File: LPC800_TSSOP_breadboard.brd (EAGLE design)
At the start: 30.5 x 17.8 mm, 16 parts, among them Q1 12MHz

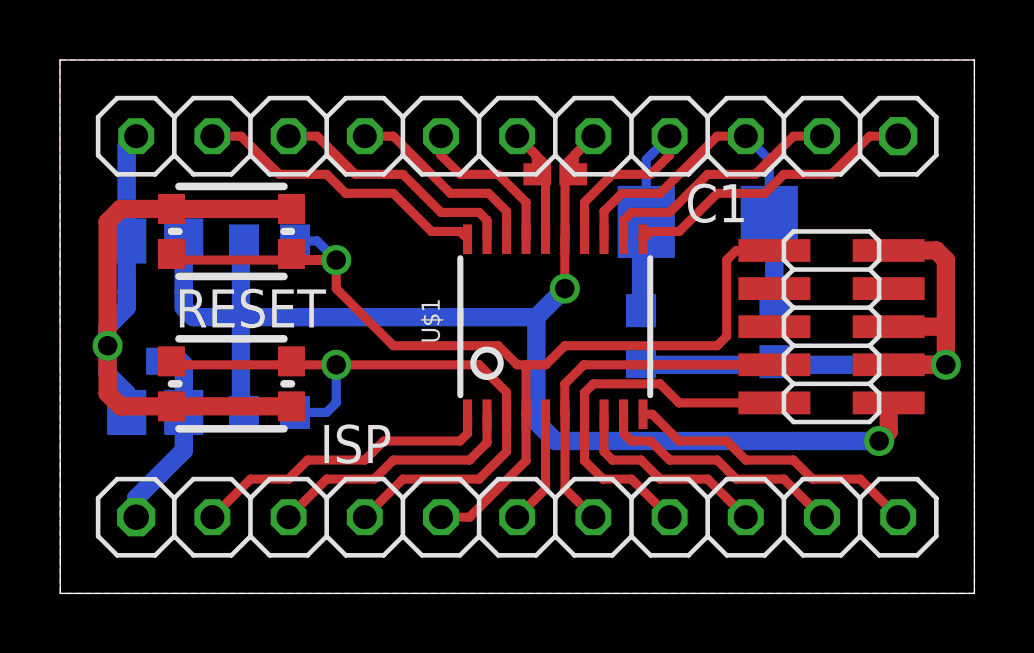
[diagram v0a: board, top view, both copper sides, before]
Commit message: * small updates
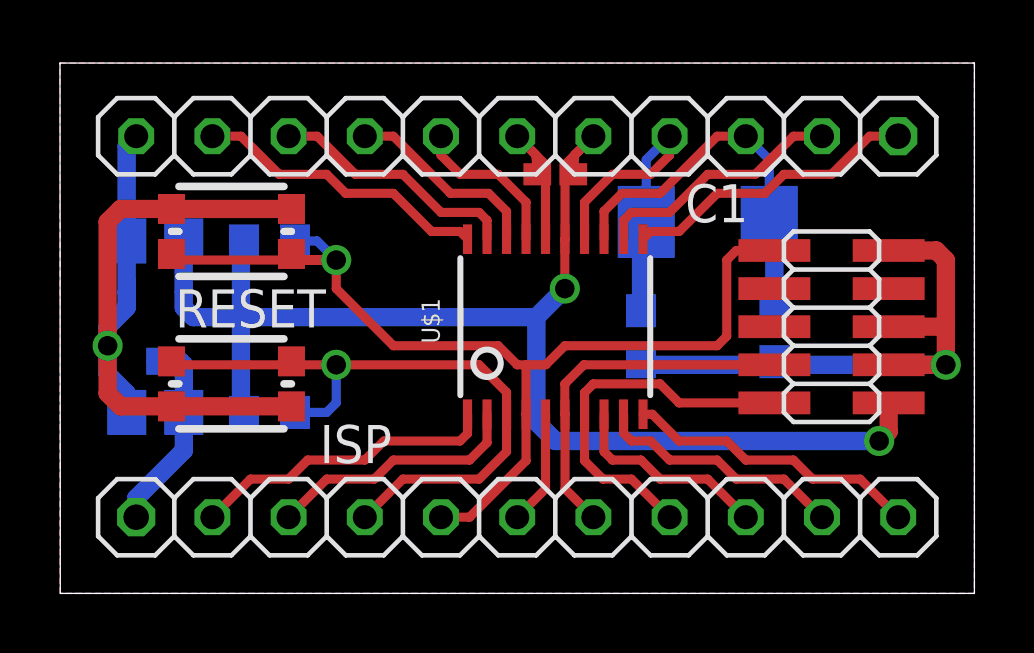
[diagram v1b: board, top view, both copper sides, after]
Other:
- board size 30.5 x 17.8 mm -> 30.5 x 17.7 mm
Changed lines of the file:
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@@
 <board>
 <plain>
-<wire x1="30.48" y1="0" x2="30.48" y2="17.78" width="0" layer="20"/>
-<wire x1="30.48" y1="17.78" x2="0" y2="17.78" width="0" layer="20"/>
-<wire x1="0" y1="17.78" x2="0.01" y2="0" width="0" layer="20"/>
+<wire x1="30.48" y1="0" x2="30.48" y2="17.6784" width="0" layer="20"/>
+<wire x1="30.48" y1="17.6784" x2="0" y2="17.6784" width="0" layer="20"/>
+<wire x1="0" y1="17.6784" x2="0.01" y2="0" width="0" layer="20"/>
 <wire x1="0.01" y1="0" x2="30.48" y2="0" width="0" layer="20"/>
 <wire x1="0" y1="0" x2="0" y2="17.6784" width="0.254" layer="102"/>
@@
 <wire x1="15.86" y1="14.62" x2="15.24" y2="15.24" width="0.3048" layer="1"/>
 <polygon width="0.254" layer="1">
-<vertex x="0" y="17.78"/>
-<vertex x="30.48" y="17.78"/>
+<vertex x="0" y="17.6784"/>
+<vertex x="30.48" y="17.6784"/>
 <vertex x="30.48" y="0"/>
 <vertex x="0" y="0"/>
 </polygon>
 <polygon width="0.254" layer="16">
-<vertex x="0" y="17.78"/>
-<vertex x="30.48" y="17.78"/>
+<vertex x="0" y="17.6784"/>
+<vertex x="30.48" y="17.6784"/>
 <vertex x="30.48" y="0"/>
 <vertex x="0" y="0"/>
